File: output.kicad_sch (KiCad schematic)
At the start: 32 parts, among them J1 SMA, J2 SMA, J3 SMA, J4 SMA, J5 U.Fl, T1 MABA-007159-000000, T2 MABA-007159-000000, U31 74LVC1G125, U41 74CB3Q3306

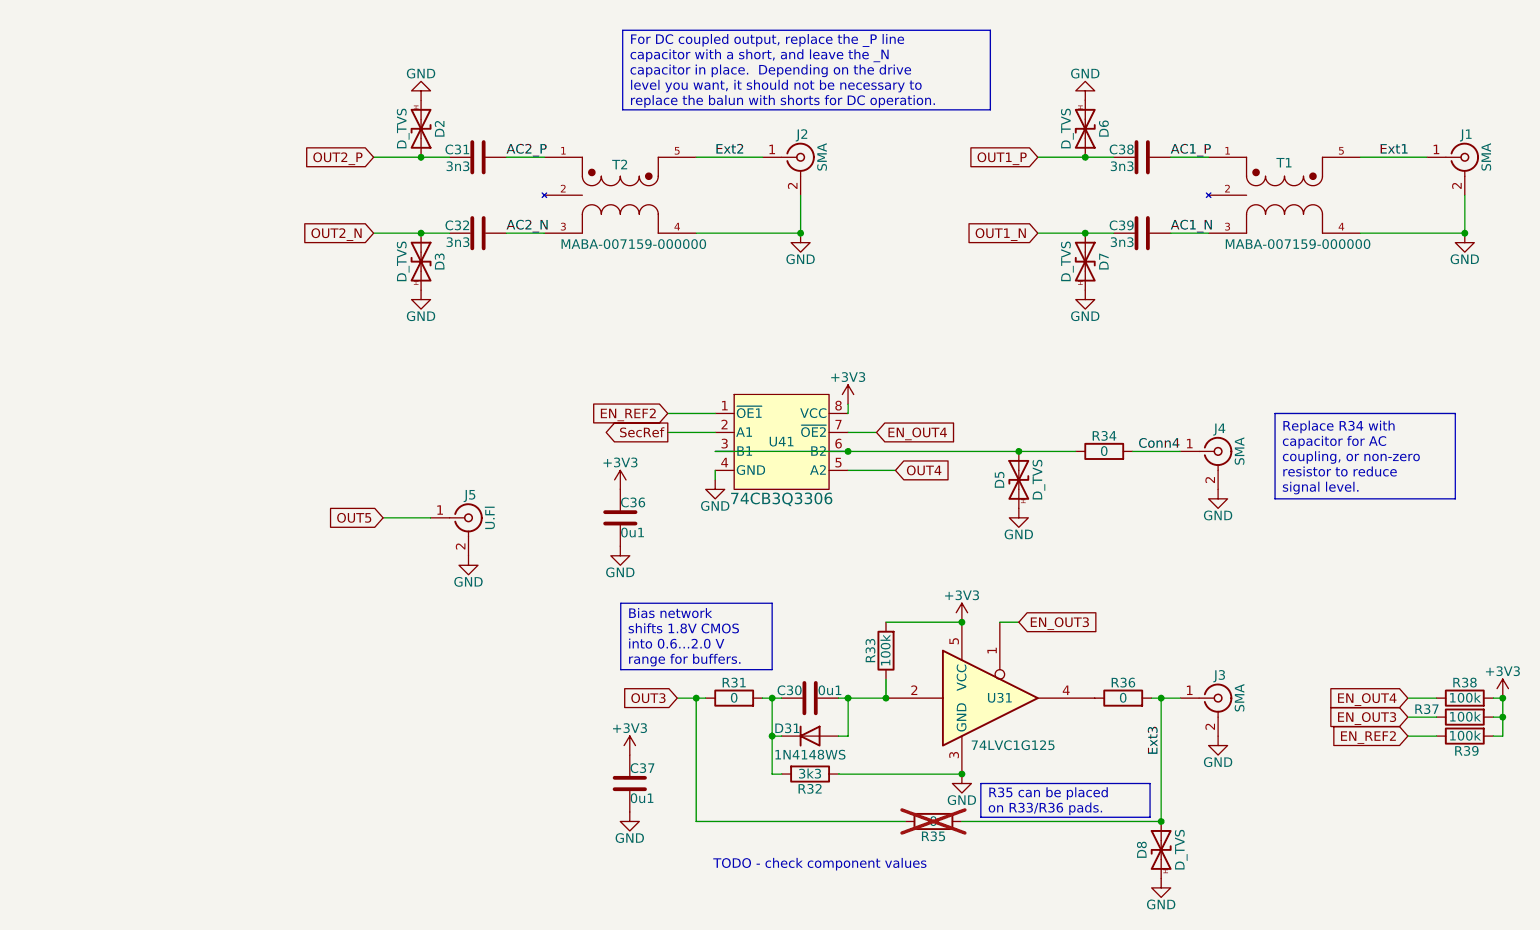
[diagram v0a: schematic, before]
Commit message: Schematic updates for revision mostly done.
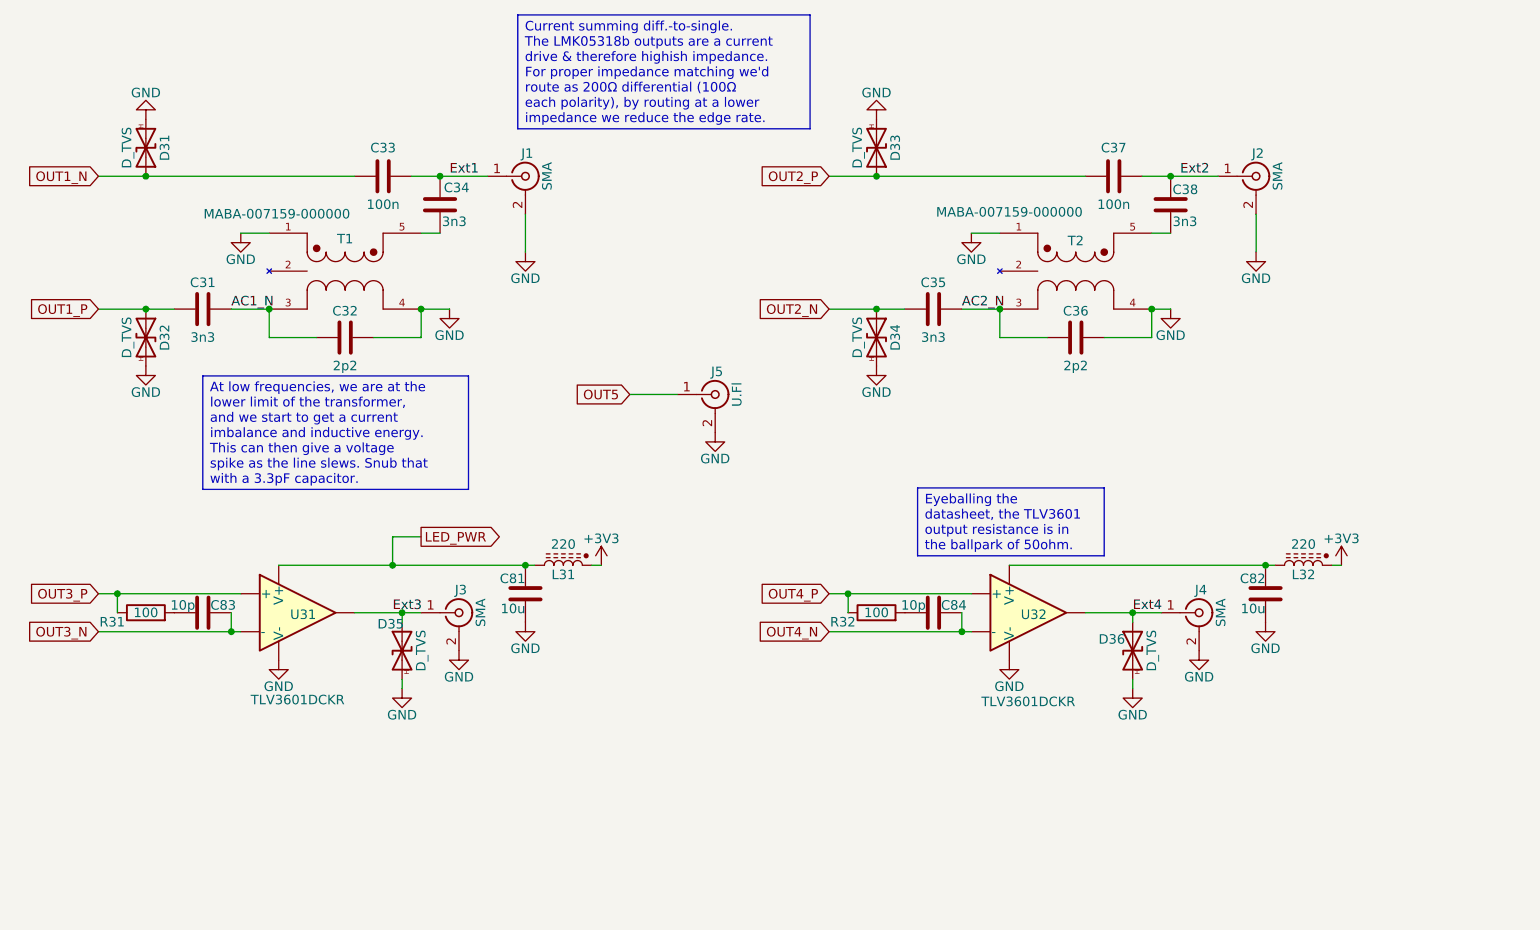
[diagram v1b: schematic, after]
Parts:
- removed C30, C37: 0u1, Capacitor_SMD:C_0402_1005Metric, symbol Device:C
- removed D31: 1N4148WS, Diode_SMD:D_SOD-323, symbol Diode:1N4148WS
- removed R33, R37, R38, R39: 100k, Resistor_SMD:R_0402_1005Metric, symbol Device:R
- removed R34, R35, R36: 0, Resistor_SMD:R_0603_1608Metric, symbol Device:R
- removed U31: 74LVC1G125, Package_TO_SOT_SMD:SOT-23-5, symbol 74xGxx:74LVC1G125
- removed U41: 74CB3Q3306, Package_SO:VSSOP-8_2.3x2mm_P0.5mm, symbol Parts:74CB3Q3306
- added C32: 2p2, Capacitor_SMD:C_0402_1005Metric, symbol Device:C
- added C33: 100n, Capacitor_SMD:C_0402_1005Metric, symbol Device:C
- added C38: 3n3, Capacitor_SMD:C_0402_1005Metric, symbol Device:C
- added C81, C82: 10u, Capacitor_SMD:C_0402_1005Metric, symbol Device:C
- added C83, C84: 10p, Capacitor_SMD:C_0402_1005Metric, symbol Device:C
- added L31, L32: 220, Inductor_SMD:L_0603_1608Metric, symbol Parts:L_Ferrite_Power
- added U31, U32: TLV3601DCKR, Package_TO_SOT_SMD:SOT-353_SC-70-5, symbol Parts:TLV3601DCKR
- C31: renamed from C39; LCSC C26404 -> (none)
- C35: renamed from C32; LCSC C26404 -> (none)
- C36: value 0u1 -> 2p2; LCSC C307331 -> (none)
- C37: renamed from C31; value 3n3 -> 100n; LCSC C26404 -> (none)
- R31: value 0 -> 100; footprint Resistor_SMD:R_0603_1608Metric -> Resistor_SMD:R_0402_1005Metric; LCSC C21189 -> C25076
- R32: value 3k3 -> 100; LCSC C25890 -> C25076
- renumbered C38 to C34, D6 to D31, D7 to D32, D2 to D33, D3 to D34, D8 to D35, D5 to D36
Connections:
- net Conn4 is gone; now on net Ext4: J4.1 (In)
- net +3V3: now also L31.1, L32.1; no longer C36.1
- net AC1_N: now also C32.1
- net AC2_N: now also C36.1
- net Ext1: now also C34.2, C33.2; no longer T1.5
- net Ext2: now also C37.2, C38.2; no longer T2.5
- net Ext3: now also U31.1
- net GND: now also T1.1, T2.1, C32.2, C81.2, C82.2, U31.2 (V-), U32.2 (V-); no longer R32.1
- net OUT1_N: now also D31.1 (A1), C33.1; no longer C31.1, D32.1 (A1)
- net OUT1_P: now also C31.1, D32.1 (A1); no longer C34.1, D31.1 (A1)
- net at R31.2: now also C83.1; no longer R32.2
- net Ext4: now reaches D36.1 (A1)
- net Ext4: now also U32.1
- removed net AC1_P: C34.2, T1.1
- removed net AC2_P: C37.2, T2.1
- net OUT3 renamed OUT3_P
- net OUT3_P: now also U31.3 (+)
- new net: C84.1, R32.2
- new net: C34.1, T1.5
- new net: C82.1, L32.2, U32.5 (V+)
- new net: C38.1, T2.5
- new net LED_PWR: C81.1, L31.2, U31.5 (V+)
- new net OUT3_N: C83.2, U31.4 (-)
- new net OUT4_N: C84.2, U32.4 (-)
- new net OUT4_P: R32.1, U32.3 (+)
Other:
- note removed: "TODO - check component values"
- moved on the sheet: C31, C34, C35, C37, D31, D32, D33, D34, D35, D36, J1, J2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
